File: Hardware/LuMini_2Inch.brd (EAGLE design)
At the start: 54.2 x 54.2 mm, 73 parts, among them J1 SOLDER_PAD_2, J2 SOLDER_PAD_2, J3 SOLDER_PAD_2

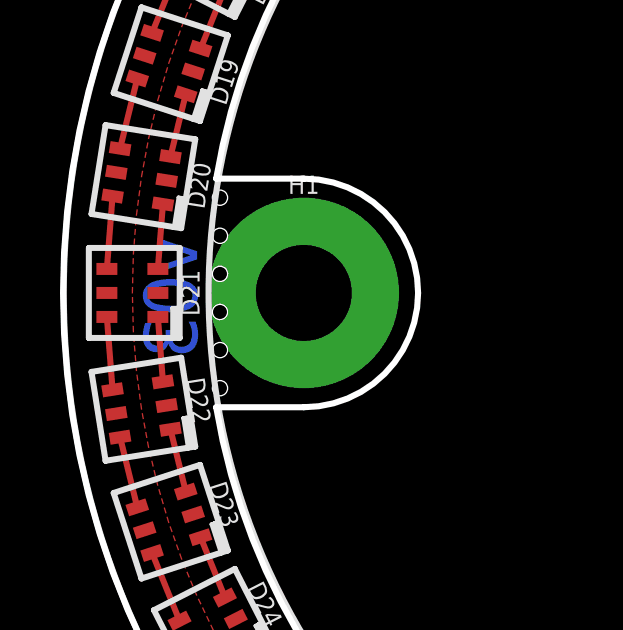
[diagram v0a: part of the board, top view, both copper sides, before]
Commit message: version number change
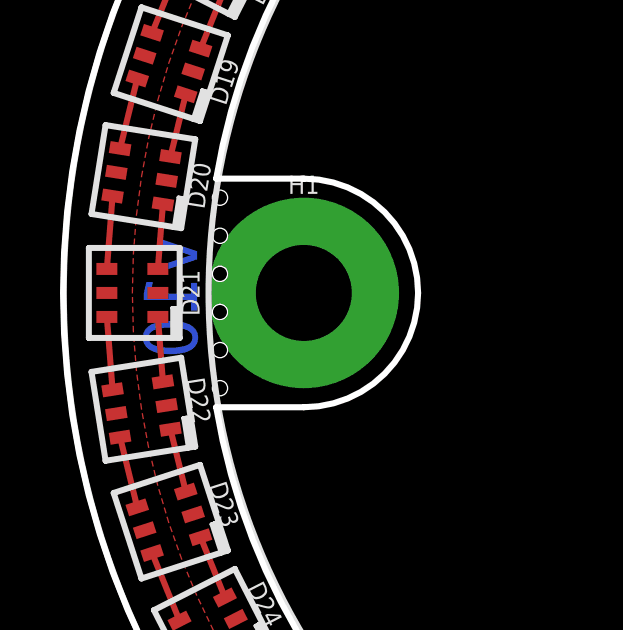
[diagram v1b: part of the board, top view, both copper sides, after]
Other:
- board text added: "v10"
- board text removed: "v03"
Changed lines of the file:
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@@
 <plain>
 <circle x="27.94" y="27.94" radius="27.051" width="0.2032" layer="21"/>
-<text x="5.334" y="29.845" size="1.778" layer="16" font="vector" ratio="15" rot="SMR270">v03</text>
+<text x="5.334" y="29.845" size="1.778" layer="16" font="vector" ratio="15" rot="SMR270">v10</text>
 <hole x="49.784" y="27.305" drill="0.508"/>
 <wire x1="5.969" y1="31.75" x2="8.89" y2="31.75" width="0.2032" layer="20"/>
